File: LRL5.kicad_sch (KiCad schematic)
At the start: 32 parts, among them J1 POWER, J2 On/Off, J5 OUT, J6 MODE, J7 DEBUG, J8 BTN, Q1 BC549, U1 BA033CC0T, U2 NHD-C0220BIZ

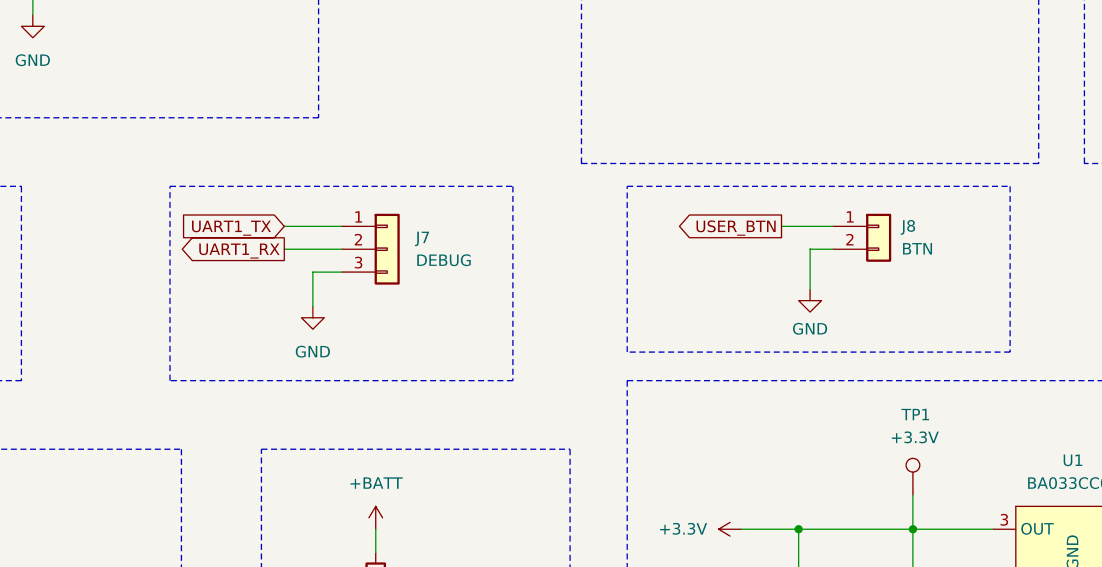
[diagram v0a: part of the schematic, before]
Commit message: Add profuction files
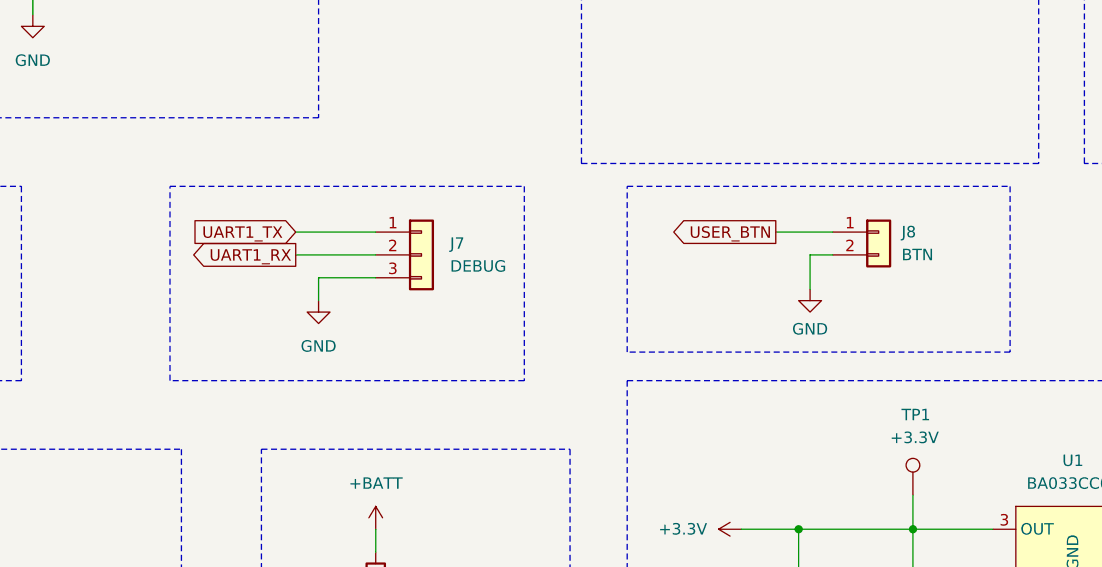
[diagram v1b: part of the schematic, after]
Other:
- moved on the sheet: J7, J8
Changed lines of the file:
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@@
 	(wire
 		(pts
+			(xy 168.91 93.98) (xy 175.26 93.98)
+		)
+		(stroke
+			(width 0)
+			(type default)
+		)
+	)
+	(wire
+		(pts
 			(xy 44.45 144.78) (xy 46.99 144.78)
 		)
@@
 	(wire
 		(pts
+			(xy 115.57 93.98) (xy 124.46 93.98)
+		)
+		(stroke
+			(width 0)
+			(type default)
+		)
+	)
+	(wire
+		(pts
 			(xy 184.15 139.7) (xy 184.15 146.05)
 		)
@@
 	(wire
 		(pts
+			(xy 172.72 100.33) (xy 172.72 96.52)
+		)
+		(stroke
+			(width 0)
+			(type default)
+		)
+	)
+	(wire
+		(pts
 			(xy 44.45 144.78) (xy 44.45 153.67)
 		)
@@
 	(wire
 		(pts
+			(xy 124.46 99.06) (xy 118.11 99.06)
+		)
+		(stroke
+			(width 0)
+			(type default)
+		)
+	)
+	(wire
+		(pts
+			(xy 172.72 96.52) (xy 175.26 96.52)
+		)
+		(stroke
+			(width 0)
+			(type default)
+		)
+	)
+	(wire
+		(pts
 			(xy 72.39 36.83) (xy 53.34 36.83)
 		)
@@
 	(wire
 		(pts
+			(xy 115.57 96.52) (xy 124.46 96.52)
+		)
+		(stroke
+			(width 0)
+			(type default)
+		)
+	)
+	(wire
+		(pts
 			(xy 165.1 127) (xy 171.45 127)
 		)
@@
 	(wire
 		(pts
-			(xy 114.3 95.885) (xy 120.65 95.885)
-		)
-		(stroke
-			(width 0)
-			(type default)
-		)
-	)
-	(wire
-		(pts
 			(xy 229.87 127) (xy 233.68 127)
 		)
@@
 	(wire
 		(pts
-			(xy 114.3 93.345) (xy 120.65 93.345)
-		)
-		(stroke
-			(width 0)
-			(type default)
-		)
-	)
-	(wire
-		(pts
 			(xy 86.36 57.15) (xy 86.36 59.69)
 		)
@@
 	(wire
 		(pts
-			(xy 117.475 98.425) (xy 120.65 98.425)
-		)
-		(stroke
-			(width 0)
-			(type default)
-		)
-	)
-	(wire
-		(pts
 			(xy 36.83 54.61) (xy 53.34 54.61)
 		)
@@
 	(wire
 		(pts
-			(xy 175.26 95.885) (xy 172.72 95.885)
-		)
-		(stroke
-			(width 0)
-			(type default)
-		)
-	)
-	(wire
-		(pts
 			(xy 255.27 34.29) (xy 259.08 34.29)
 		)
@@
 	(wire
 		(pts
-			(xy 117.475 102.235) (xy 117.475 98.425)
-		)
-		(stroke
-			(width 0)
-			(type default)
-		)
-	)
-	(wire
-		(pts
 			(xy 255.27 69.85) (xy 260.35 69.85)
 		)
@@
 	(wire
 		(pts
-			(xy 169.545 93.345) (xy 175.26 93.345)
+			(xy 201.93 146.05) (xy 201.93 149.86)
 		)
 		(stroke
@@
 	(wire
 		(pts
-			(xy 201.93 146.05) (xy 201.93 149.86)
+			(xy 118.11 99.06) (xy 118.11 101.6)
 		)
 		(stroke
@@
 	(wire
 		(pts
-			(xy 172.72 95.885) (xy 172.72 100.33)
-		)
-		(stroke
-			(width 0)
-			(type default)
-		)
-	)
-	(wire
-		(pts
 			(xy 255.27 41.91) (xy 260.35 41.91)
 		)
@@
 	(rectangle
 		(start 101.6 88.9)
-		(end 139.7 110.49)
+		(end 140.97 110.49)
 		(stroke
 			(width 0)
@@
 	(global_label "USER_BTN"
 		(shape output)
-		(at 169.545 93.345 180)
+		(at 168.91 93.98 180)
 		(fields_autoplaced yes)
 		(effects
@@
 		)
 		(property "Intersheetrefs" "${INTERSHEET_REFS}"
-			(at 157.0651 93.345 0)
+			(at 156.4301 93.98 0)
 			(effects
 				(font
@@
 	(global_label "UART1_RX"
 		(shape output)
-		(at 114.3 95.885 180)
+		(at 115.57 96.52 180)
 		(fields_autoplaced yes)
 		(effects
@@
 		)
 		(property "Intersheetrefs" "${INTERSHEET_REFS}"
-			(at 102.0015 95.885 0)
+			(at 103.2715 96.52 0)
 			(effects
 				(font
@@
 	(global_label "UART1_TX"
 		(shape input)
-		(at 114.3 93.345 180)
+		(at 115.57 93.98 180)
 		(fields_autoplaced yes)
 		(effects
@@
 		)
 		(property "Intersheetrefs" "${INTERSHEET_REFS}"
-			(at 102.3039 93.345 0)
+			(at 103.5739 93.98 0)
 			(effects
 				(font
@@
 	(symbol
 		(lib_id "power:GND")
-		(at 117.475 102.235 0)
+		(at 118.11 101.6 0)
 		(unit 1)
 		(exclude_from_sim no)
@@
 		(fields_autoplaced yes)
 		(property "Reference" "#PWR013"
-			(at 117.475 108.585 0)
+			(at 118.11 107.95 0)
 			(effects
 				(font
@@
 		)
 		(property "Value" "GND"
-			(at 117.475 107.315 0)
+			(at 118.11 106.68 0)
 			(effects
 				(font
@@
 		)
 		(property "Footprint" ""
-			(at 117.475 102.235 0)
+			(at 118.11 101.6 0)
 			(effects
 				(font
@@
 		)
 		(property "Datasheet" ""
-			(at 117.475 102.235 0)
+			(at 118.11 101.6 0)
 			(effects
 				(font
@@
 		)
 		(property "Description" "Power symbol creates a global label with name \"GND\" , ground"
-			(at 117.475 102.235 0)
+			(at 118.11 101.6 0)
 			(effects
 				(font
@@
 	(symbol
 		(lib_id "Connector_Generic:Conn_01x02")
-		(at 180.34 93.345 0)
+		(at 180.34 93.98 0)
 		(unit 1)
 		(exclude_from_sim no)
@@
 		(fields_autoplaced yes)
 		(property "Reference" "J8"
-			(at 182.88 93.3449 0)
+			(at 182.88 93.9799 0)
 			(effects
 				(font
@@
 		)
 		(property "Value" "BTN"
-			(at 182.88 95.8849 0)
+			(at 182.88 96.5199 0)
 			(effects
 				(font
@@
 		)
 		(property "Footprint" "Connector_PinHeader_2.54mm:PinHeader_1x02_P2.54mm_Vertical_SMD_Pin1Left"
-			(at 180.34 93.345 0)
+			(at 180.34 93.98 0)
 			(effects
 				(font
@@
 		)
 		(property "Datasheet" "~"
-			(at 180.34 93.345 0)
+			(at 180.34 93.98 0)
 			(effects
 				(font
@@
 		)
 		(property "Description" "Generic connector, single row, 01x02, script generated (kicad-library-utils/schlib/autogen/connector/)"
-			(at 180.34 93.345 0)
+			(at 180.34 93.98 0)
 			(effects
 				(font
@@
 	(symbol
 		(lib_id "Connector_Generic:Conn_01x03")
-		(at 125.73 95.885 0)
+		(at 129.54 96.52 0)
 		(unit 1)
 		(exclude_from_sim no)
@@
 		(fields_autoplaced yes)
 		(property "Reference" "J7"
-			(at 128.905 94.6149 0)
+			(at 132.715 95.2499 0)
 			(effects
 				(font
@@
 		)
 		(property "Value" "DEBUG"
-			(at 128.905 97.1549 0)
+			(at 132.715 97.7899 0)
 			(effects
 				(font
@@
 		)
 		(property "Footprint" "Connector_PinHeader_2.54mm:PinHeader_1x03_P2.54mm_Vertical_SMD_Pin1Left"
-			(at 125.73 95.885 0)
+			(at 129.54 96.52 0)
 			(effects
 				(font
@@
 		)
 		(property "Datasheet" "~"
-			(at 125.73 95.885 0)
+			(at 129.54 96.52 0)
 			(effects
 				(font
@@
 		)
 		(property "Description" "Generic connector, single row, 01x03, script generated (kicad-library-utils/schlib/autogen/connector/)"
-			(at 125.73 95.885 0)
+			(at 129.54 96.52 0)
 			(effects
 				(font
